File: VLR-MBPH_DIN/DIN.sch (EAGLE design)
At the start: 24 parts, among them IC1 74HC165NDIL16, IC2 74HC165NDIL16, IC3 74HC165NDIL16, IC4 74HC165NDIL16

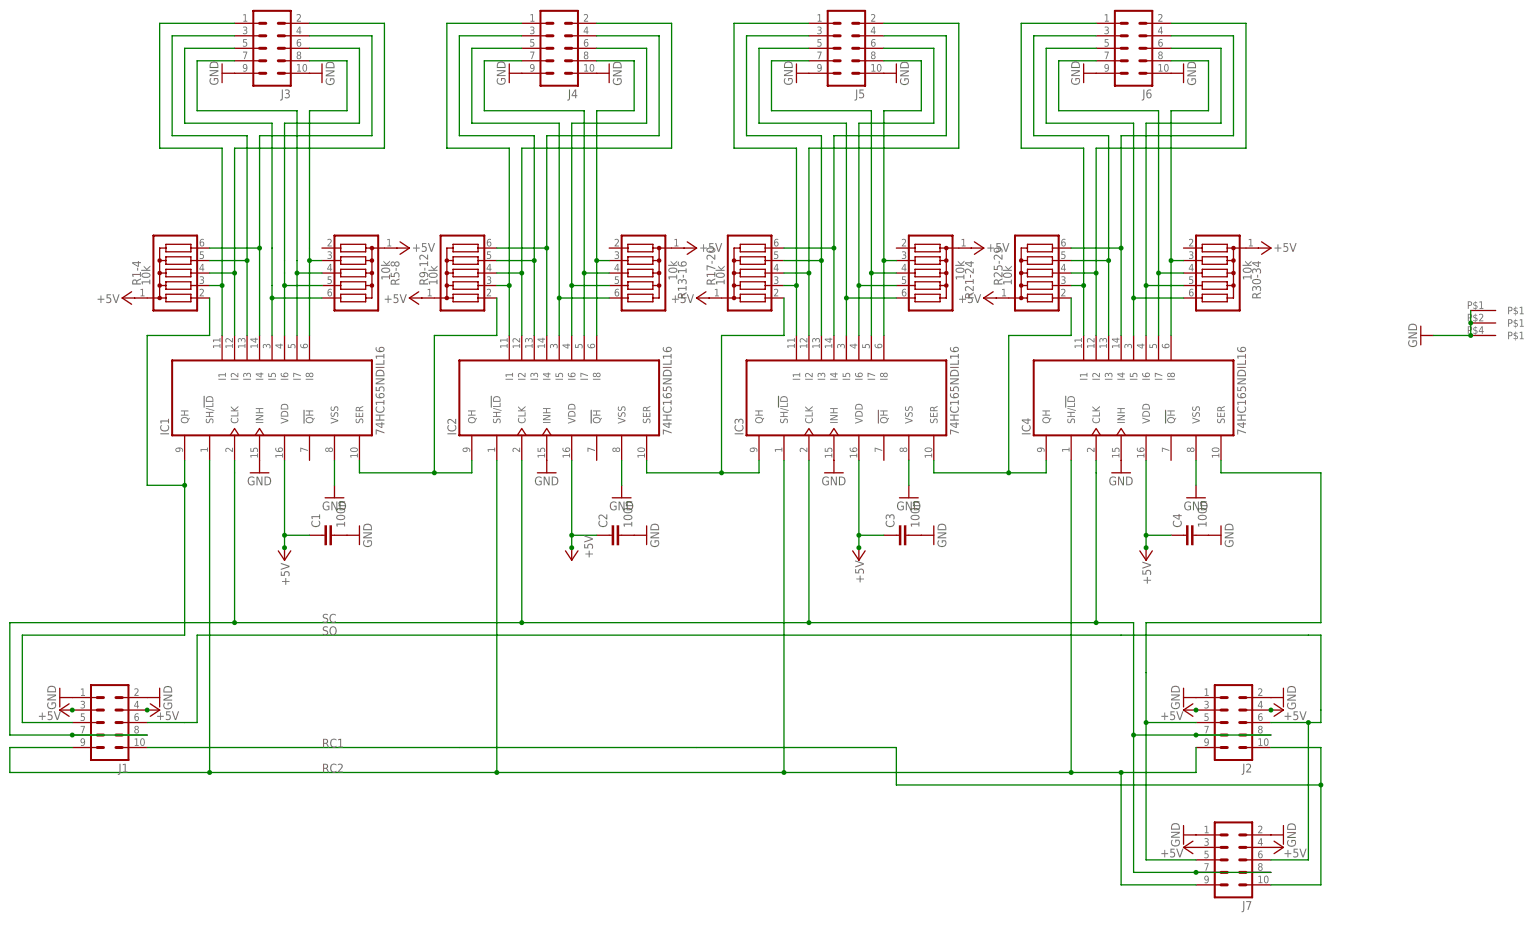
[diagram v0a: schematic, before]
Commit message: update DINv2.2
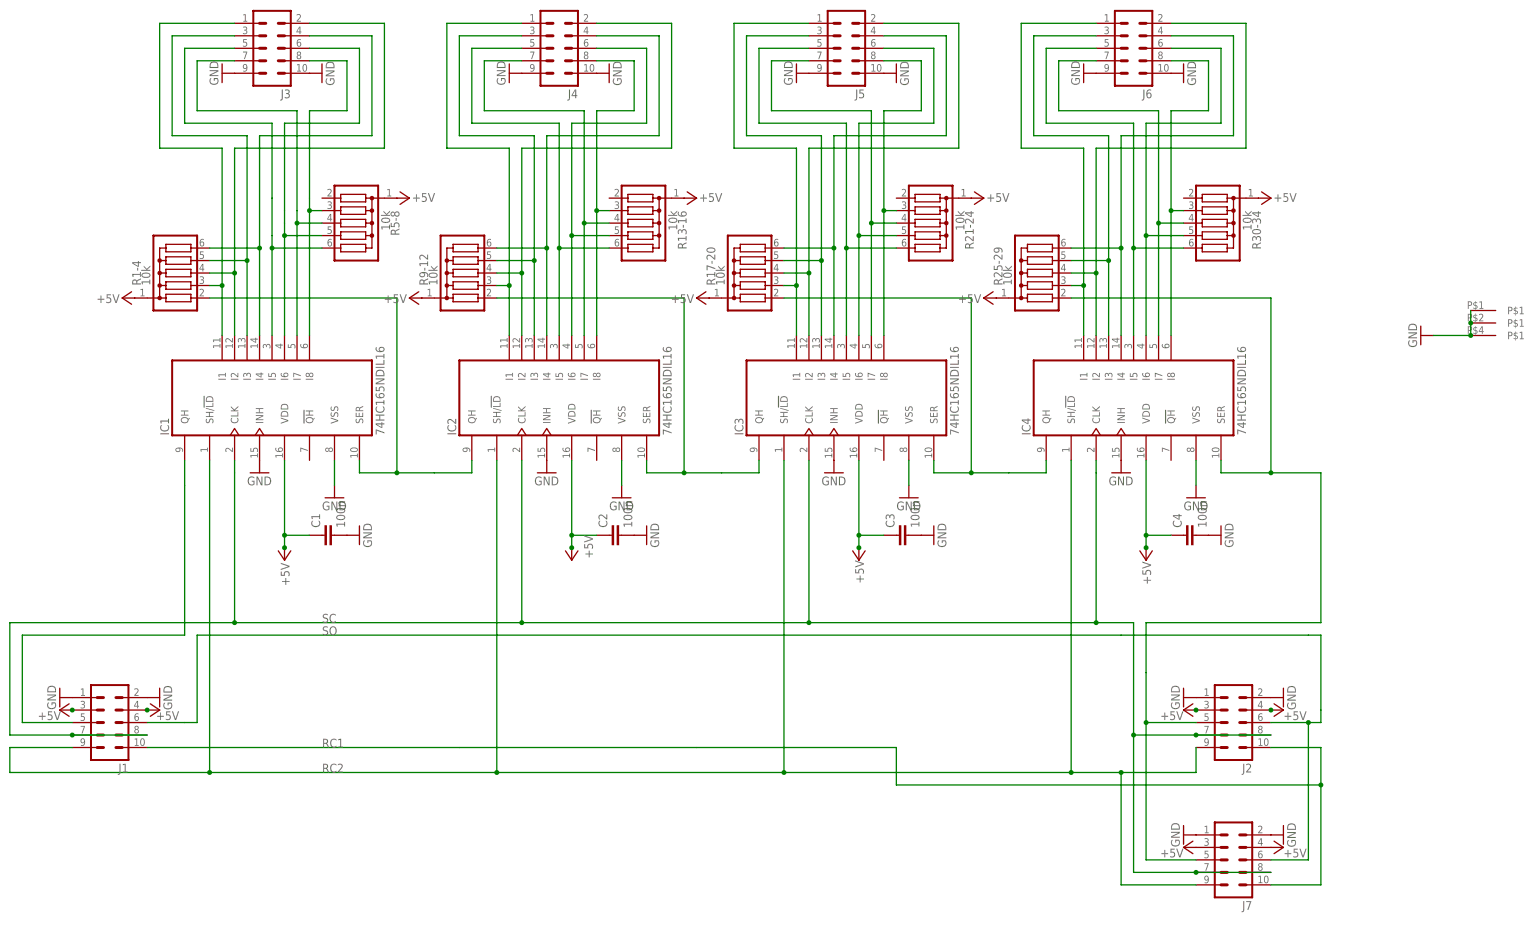
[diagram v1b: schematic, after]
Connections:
- net N$67: now also R1-4.2; no longer R9-12.2
- net N$68: now also R9-12.2; no longer R17-20.2
- net N$69: now also R17-20.2; no longer R25-29.2
- net SI: no longer R1-4.2
- net SI2: now also R25-29.2
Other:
- moved on the sheet: R13-16, R21-24, R30-34, R5-8
